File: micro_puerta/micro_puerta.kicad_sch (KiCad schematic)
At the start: 13 parts, among them J1 Entrada NPN, J10 Screw_Terminal_01x02, J11 Screw_Terminal_01x02, J12 Screw_Terminal_01x02, J13 Screw_Terminal_01x02, J2 Entradas PNP, J3 Entrada An 0-32V, J4 Entrada An 0-10V, J5 Relay, J6 Entrada An 4-20mA, J7 Salida An 4-20mA, J8 Salida An 0-10V, J9 RS485

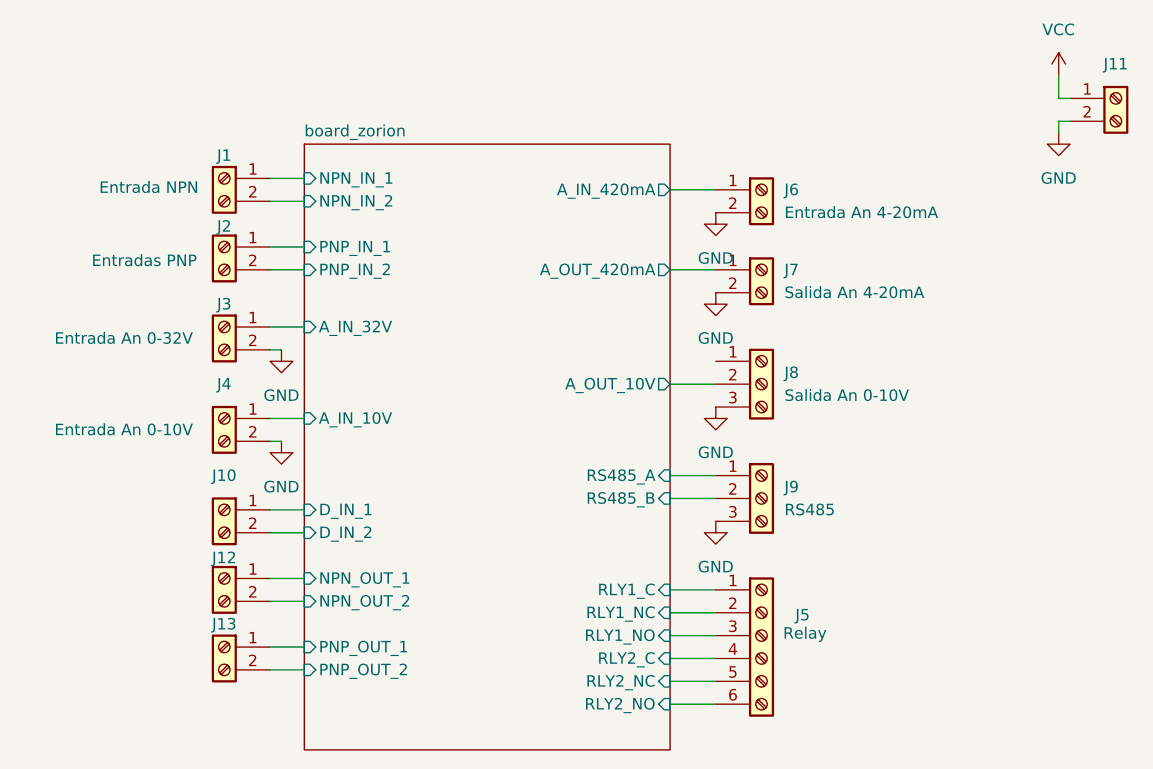
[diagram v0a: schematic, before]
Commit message: nueva actualizacion
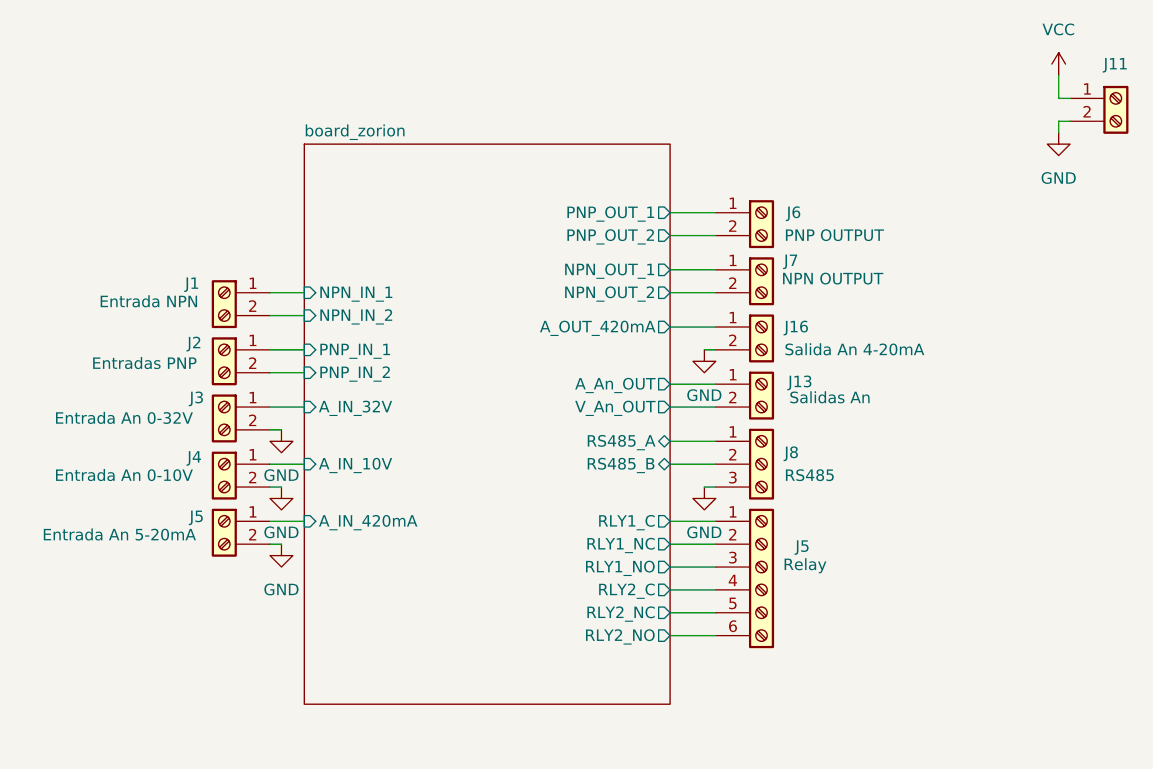
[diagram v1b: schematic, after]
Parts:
- removed J8: Salida An 0-10V, TerminalBlock_Phoenix:TerminalBlock_Phoenix_MKDS-1,5-3-5.08_1x03_P5.08mm_Horizontal, symbol Connector:Screw_Terminal_01x03
- J13: value Screw_Terminal_01x02 -> Salidas An
- J5: renamed from J12; value Screw_Terminal_01x02 -> Entrada An 5-20mA
- J6: value Entrada An 4-20mA -> PNP OUTPUT
- J7: renamed from J10; value Screw_Terminal_01x02 -> NPN OUTPUT
- renumbered J7 to J16, J9 to J8
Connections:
- net board_zorion/D_IN_1 is gone; now on net board_zorion/NPN_OUT_1: J7.1 (Pin_1)
- net board_zorion/D_IN_2 is gone; now on net board_zorion/NPN_OUT_2: J7.2 (Pin_2)
- net GND: now also J5.2 (Pin_2); no longer J6.2 (Pin_2)
- net board_zorion/A_IN_420mA: now also J5.1 (Pin_1); no longer J6.1 (Pin_1)
- net board_zorion/NPN_OUT_1: no longer J5.1 (Pin_1)
- net board_zorion/NPN_OUT_2: no longer J5.2 (Pin_2)
- net board_zorion/PNP_OUT_1: now also J6.1 (Pin_1); no longer J13.1 (Pin_1)
- net board_zorion/PNP_OUT_2: now also J6.2 (Pin_2); no longer J13.2 (Pin_2)
- new net board_zorion/A_An_OUT: J13.1 (Pin_1)
- new net board_zorion/V_An_OUT: J13.2 (Pin_2)
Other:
- sheet board_zorion ports: added A_An_OUT, V_An_OUT; removed A_OUT_10V, D_IN_1, D_IN_2
- moved on the sheet: J1, J13, J16, J2, J3, J4, J5, J6, J7, J8
